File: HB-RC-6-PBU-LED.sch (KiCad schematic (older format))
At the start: 43 parts, among them IC1 CC1101, J1 Screw_Terminal_01x02, J2 ISP, J3 FTDI, Q1 IRLML9301, SW1 Config, SW2 BTN1, SW3 BTN2, SW4 BTN3, SW5 BTN4, SW6 BTN5, SW7 BTN6, U1 ATmega644A-AU, U2 TLV1117-33, U3 SN74LVC1T45DBV

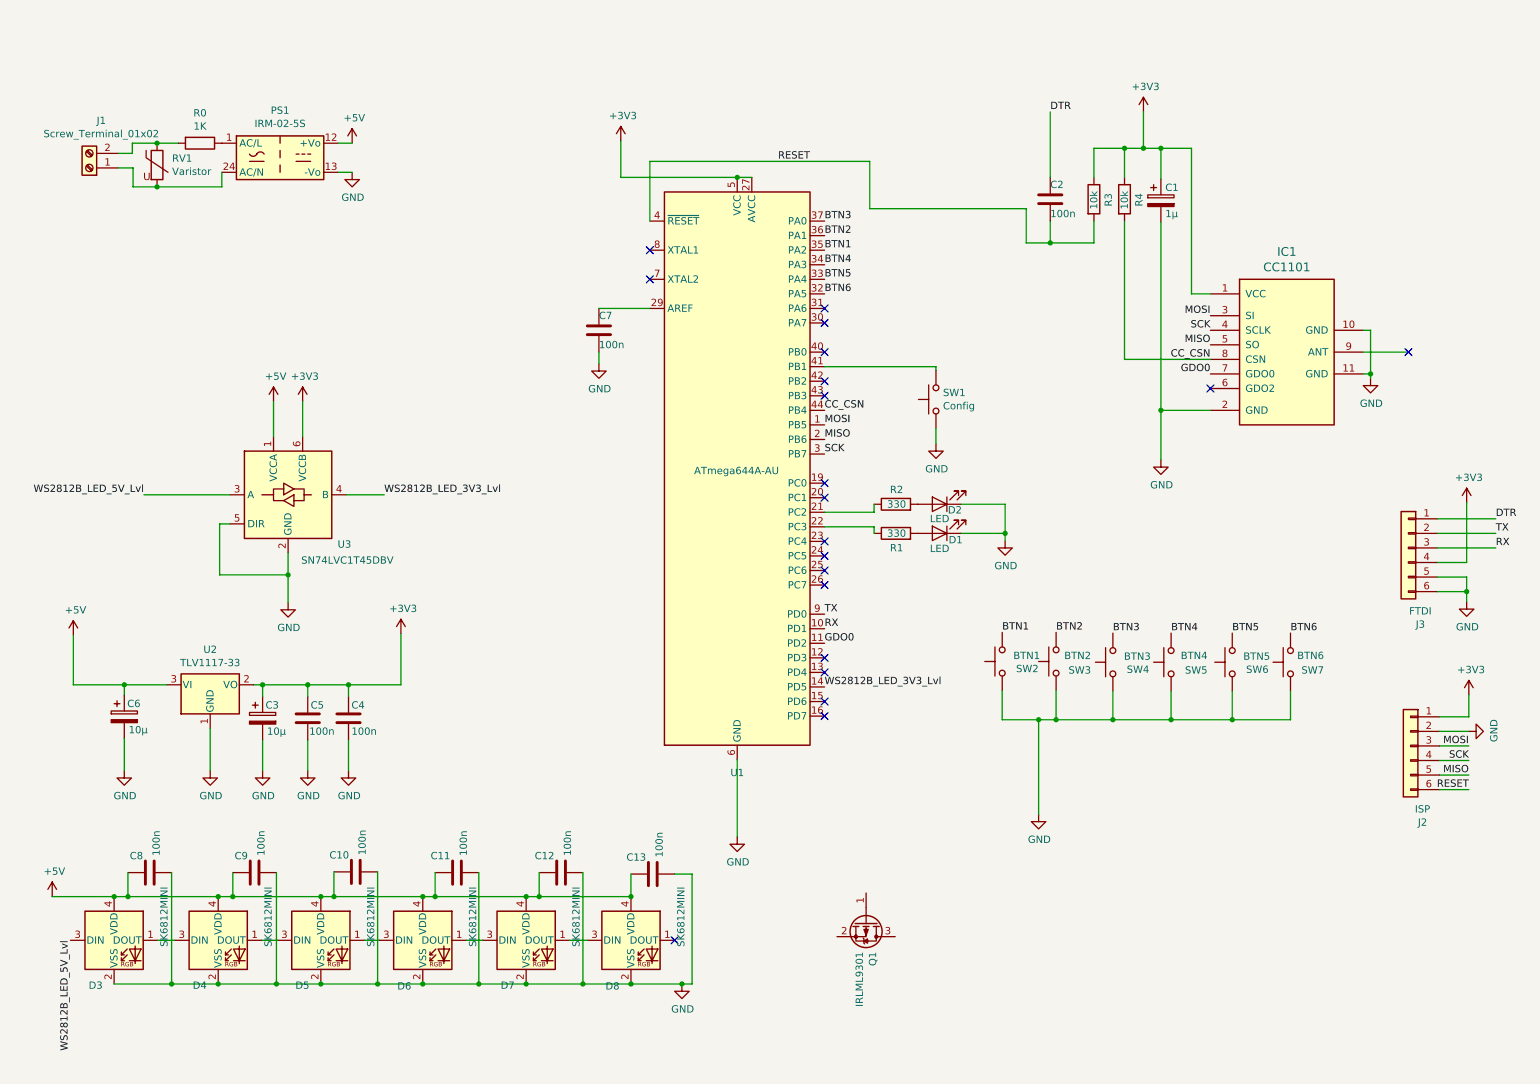
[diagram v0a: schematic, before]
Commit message: Add files via upload
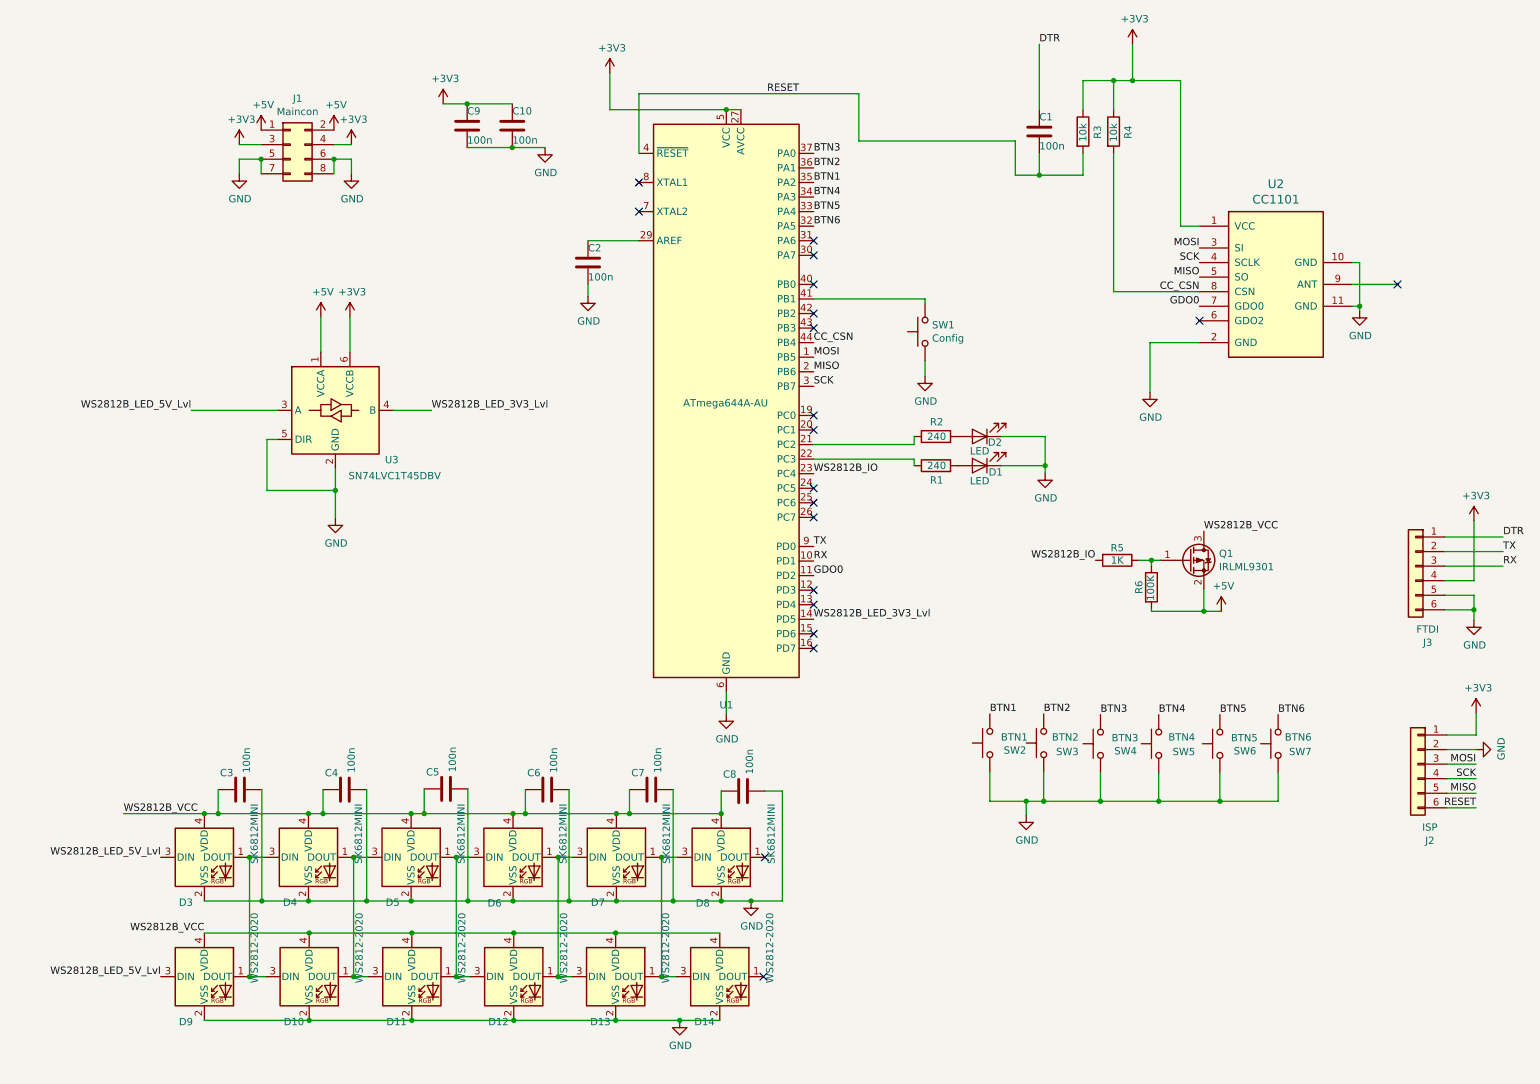
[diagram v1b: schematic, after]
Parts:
- removed C1: 1µ, Capacitor_SMD:CP_Elec_4x5.3, symbol Device:CP
- removed C3, C6: 10µ, Capacitor_SMD:CP_Elec_4x5.4, symbol Device:CP
- removed C4, C5: 100n, Capacitor_SMD:C_0805_2012Metric_Pad1.18x1.45mm_HandSolder, symbol Device:C
- removed J1: Screw_Terminal_01x02, symbol Connector:Screw_Terminal_01x02
- removed PS1: IRM-02-5S, Converter_ACDC:Converter_ACDC_MeanWell_IRM-02-xx_SMD, symbol Converter_ACDC:IRM-02-5S
- removed R0: 1K, Resistor_THT:R_Axial_DIN0204_L3.6mm_D1.6mm_P2.54mm_Vertical, symbol Device:R
- removed RV1: Varistor, Varistor:RV_Disc_D7mm_W3.4mm_P5mm, symbol Device:Varistor
- removed U2: TLV1117-33, Package_TO_SOT_SMD:SOT-223, symbol Regulator_Linear:TLV1117-33
- added C10, C9: 100n, Capacitor_SMD:C_0805_2012Metric_Pad1.18x1.45mm_HandSolder, symbol Device:C
- added D10, D11, D12, D13, D14, D9: WS2812-2020, WS2812-2020:LED_WS2812-2020, symbol LED:SK6812MINI
- added J1: Maincon, Connector_PinHeader_2.54mm:PinHeader_2x04_P2.54mm_Vertical_SMD, symbol Connector_Generic:Conn_02x04_Odd_Even
- added R5: 1K, Resistor_SMD:R_0805_2012Metric_Pad1.20x1.40mm_HandSolder, symbol Device:R
- added R6: 100K, Resistor_SMD:R_0805_2012Metric_Pad1.20x1.40mm_HandSolder, symbol Device:R
- R1, R2: value 330 -> 240
- renumbered C2 to C1, C7 to C2, C8 to C3, C9 to C4, C10 to C5, C11 to C6, C12 to C7, C13 to C8, IC1 to U2
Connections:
- net +3V3: now also C10.1, C9.1, J1.3 (Pin_3), J1.4 (Pin_4)
- net +5V: now also Q1.2 (S), J1.1 (Pin_1), J1.2 (Pin_2), R6.2; no longer C3.2, C4.2, C5.2, C6.2, C7.2, C8.2, D3.4 (VDD), D4.4 (VDD), D5.4 (VDD), D6.4 (VDD), D7.4 (VDD), D8.4 (VDD)
- net GND: now also C10.2, C9.2, D10.2 (VSS), D11.2 (VSS), D12.2 (VSS), D13.2 (VSS), D14.2 (VSS), D9.2 (VSS), J1.5 (Pin_5), J1.6 (Pin_6), J1.7 (Pin_7), J1.8 (Pin_8)
- net WS2812B_LED_5V_Lvl: now also D9.3 (DIN)
- net at D6.1 (DOUT), D7.3 (DIN): now also D12.1 (DOUT), D13.3 (DIN)
- net at D5.1 (DOUT), D6.3 (DIN): now also D11.1 (DOUT), D12.3 (DIN)
- net at D3.1 (DOUT), D4.3 (DIN): now also D10.3 (DIN), D9.1 (DOUT)
- net at D7.1 (DOUT), D8.3 (DIN): now also D13.1 (DOUT), D14.3 (DIN)
- net at D4.1 (DOUT), D5.3 (DIN): now also D10.1 (DOUT), D11.3 (DIN)
- net WS2812B_IO: now reaches U1.23 (PC4)
- net WS2812B_IO: now also R5.2
- net at Q1.1 (G): now also R5.1, R6.1
- net WS2812B_VCC: now reaches Q1.3 (D)
- net WS2812B_VCC: now also C3.2, C4.2, C5.2, C6.2, C7.2, C8.2, D3.4 (VDD), D4.4 (VDD), D5.4 (VDD), D6.4 (VDD), D7.4 (VDD), D8.4 (VDD), D10.4 (VDD), D11.4 (VDD), D12.4 (VDD), D13.4 (VDD), D14.4 (VDD), D9.4 (VDD)
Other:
- moved on the sheet: C1, C2, C3, C4, C5, C6, C7, C8, D1, D2, D3, D4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
